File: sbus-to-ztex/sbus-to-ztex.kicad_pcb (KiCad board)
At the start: 4 copper layers, 99.7 x 83.8 mm, 64 parts, among them J1 A2541HWR-2x6P (Pmod 2x6 F R), J2 10118194-0001LF (USB micro-B), J3 Conn_02x07_Odd_Even, J4 10029449-111RLF (HDMI A), J5 Conn_01x04_Male, J6 Conn_01x03_Male, U1 SN74CB3T16211DGGR, U10 74CB3T1G125, U2 SN74CB3T16211DGGR, U3 SN74CB3T16211DGGR, U4 74CB3T1G125, U5 TPS2051CDBV, U6 SRV05-4, U7 TPD12S016PWR, U8 PCT2075DP, X1 ASE-xxxMHz

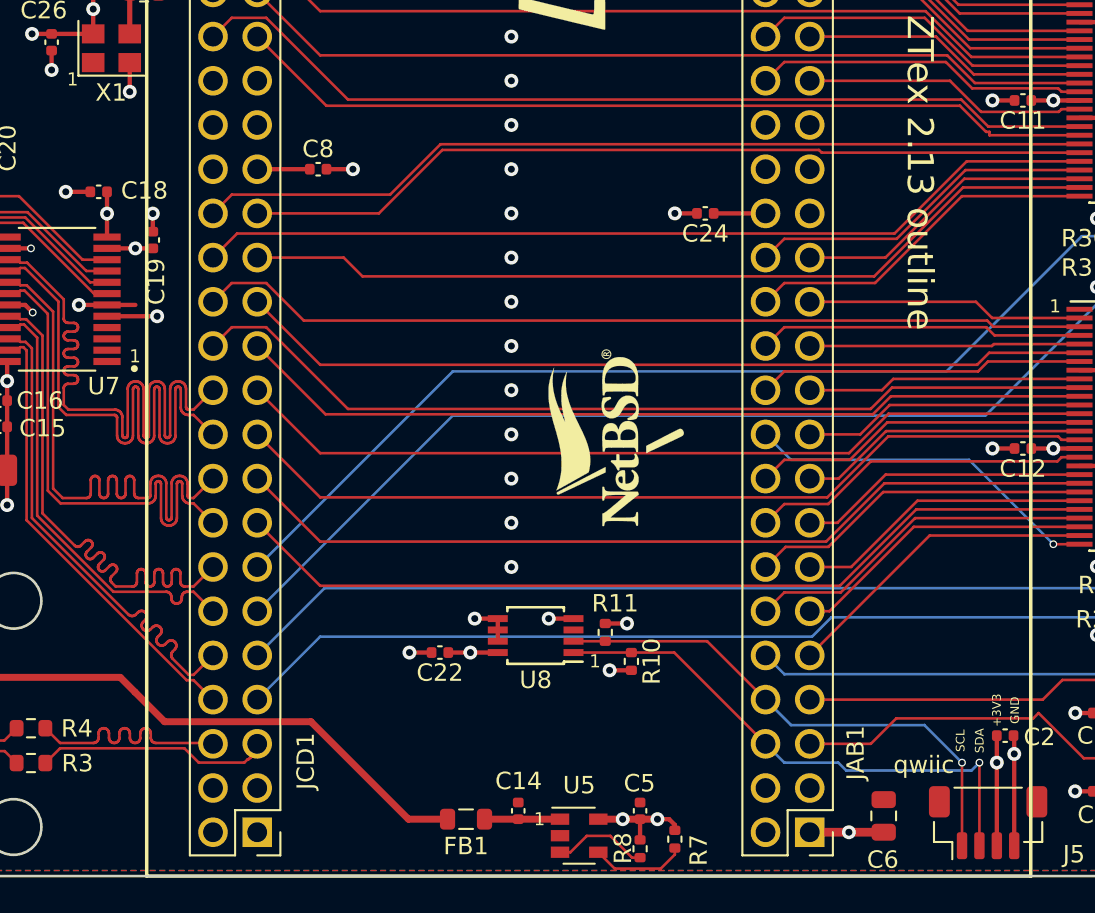
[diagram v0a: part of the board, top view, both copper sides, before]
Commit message: minor upd
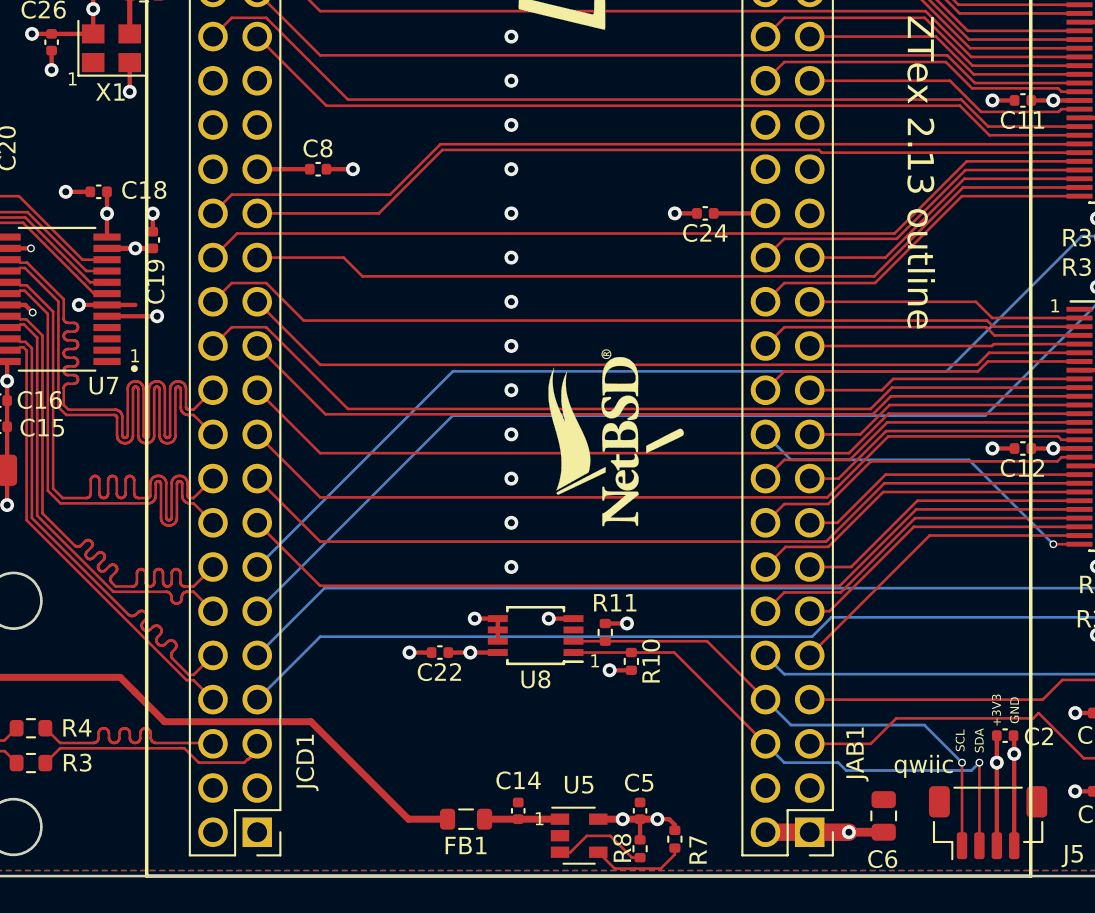
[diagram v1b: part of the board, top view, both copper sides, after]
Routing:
- net +5V: track 97.0 -> 99.6 mm
